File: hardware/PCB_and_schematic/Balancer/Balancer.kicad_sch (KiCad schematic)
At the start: 0 parts

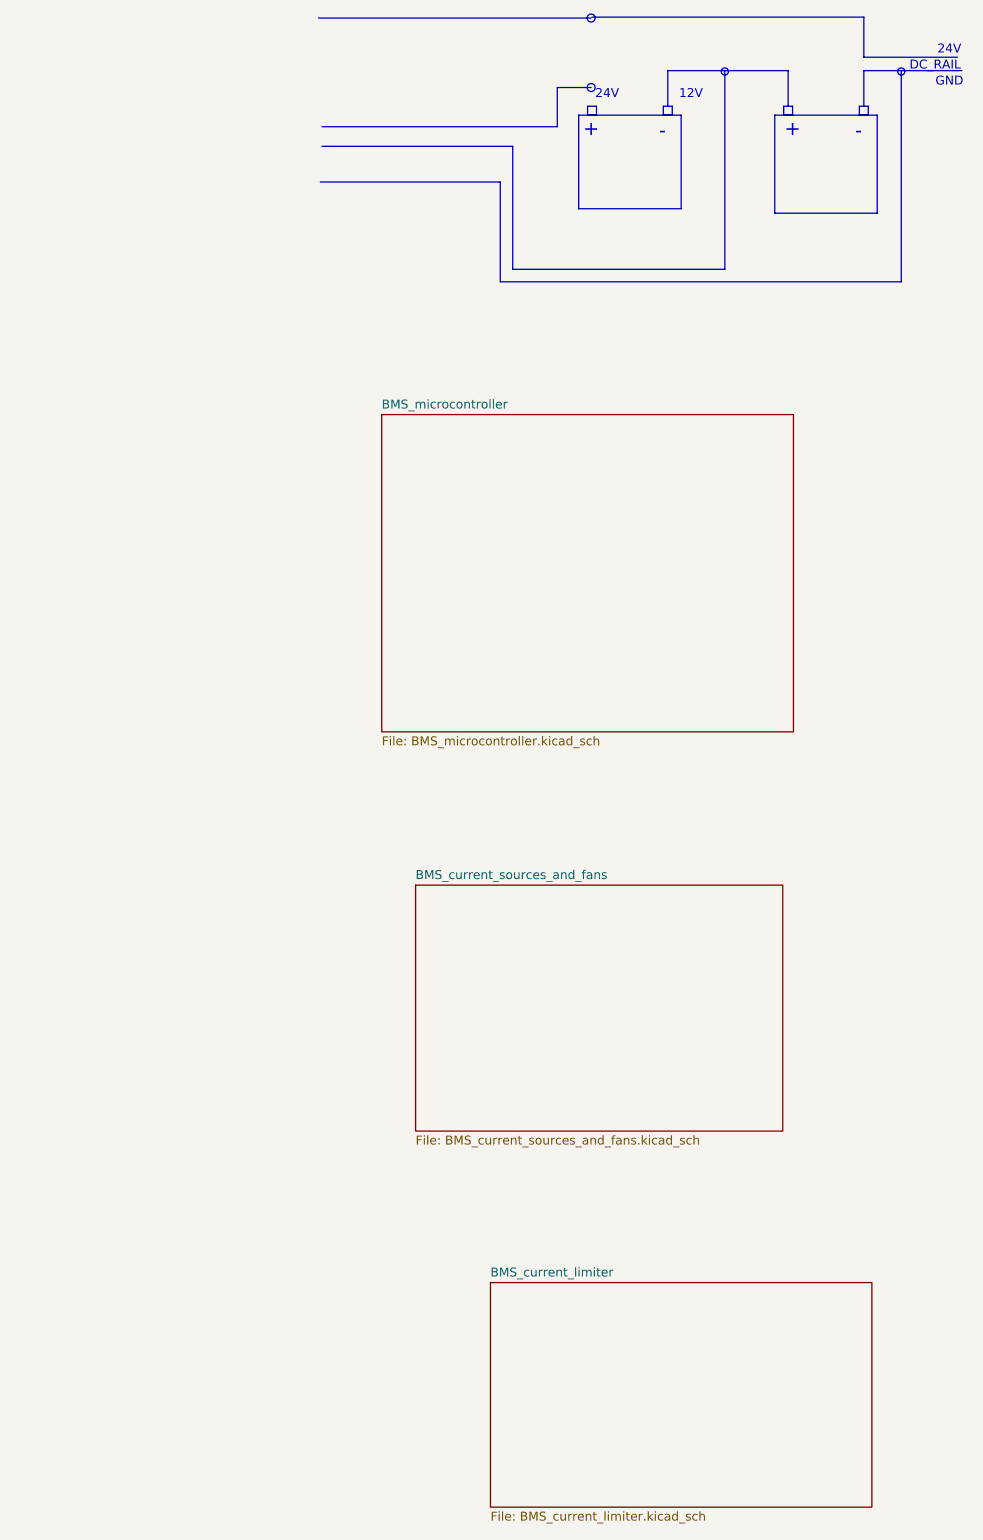
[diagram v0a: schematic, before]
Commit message: Chceck and update DC module and meter probe pcb
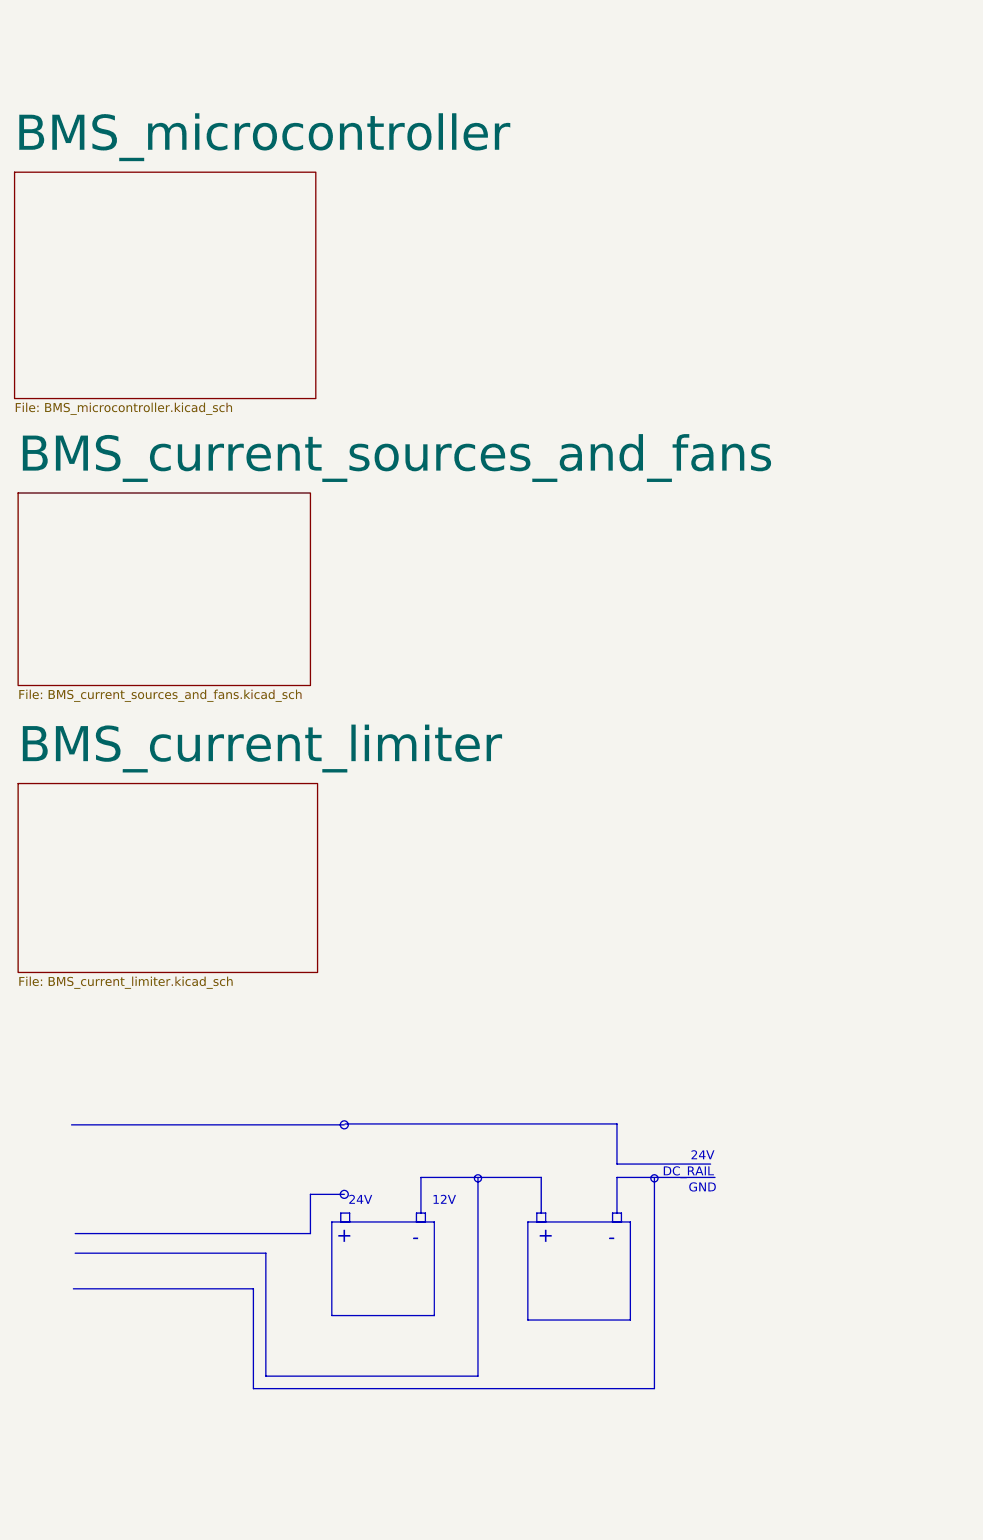
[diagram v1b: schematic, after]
